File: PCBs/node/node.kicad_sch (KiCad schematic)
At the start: 13 parts, among them J1 Bat+, J2 GND, J3 5V, SW1 SW_Push, U1 ESP32-DEVKIT-V1, U2 BME280, U3 pm25sensor, U4 lidar

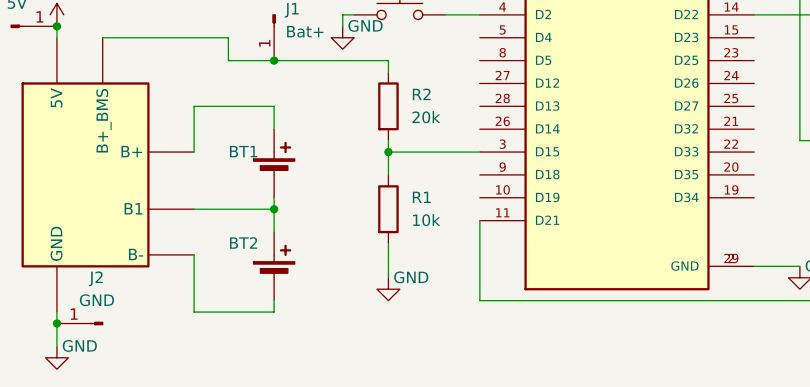
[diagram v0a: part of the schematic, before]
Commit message: changes
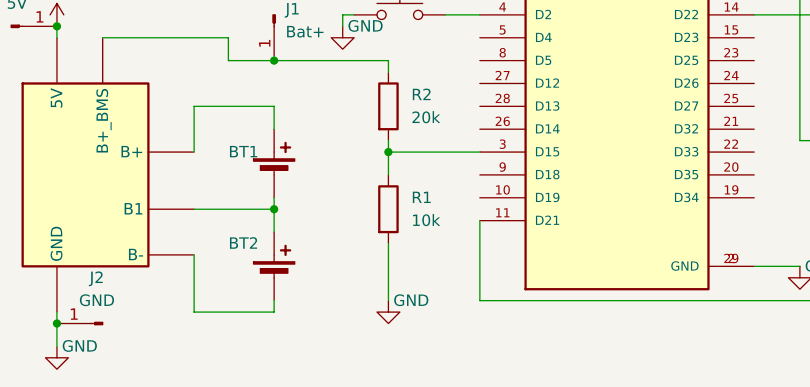
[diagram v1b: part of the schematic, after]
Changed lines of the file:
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@@
     (stroke (width 0) (type default))
   )
-  (wire (pts (xy 97.79 113.03) (xy 97.79 116.84))
+  (wire (pts (xy 97.79 113.03) (xy 97.79 119.38))
     (stroke (width 0) (type default))
   )
@@
     )
   )
-  (symbol (lib_id "power:GND") (at 97.79 116.84 0) (unit 1)
+  (symbol (lib_id "power:GND") (at 97.79 119.38 0) (unit 1)
     (in_bom yes) (on_board yes) (dnp no)
-    (property "Reference" "#PWR010" (at 97.79 123.19 0)
-      (effects (font (size 1.27 1.27)) hide)
-    )
-    (property "Value" "GND" (at 100.33 116.84 0)
-      (effects (font (size 1.27 1.27)))
-    )
-    (property "Footprint" "" (at 97.79 116.84 0)
-      (effects (font (size 1.27 1.27)) hide)
-    )
-    (property "Datasheet" "" (at 97.79 116.84 0)
-      (effects (font (size 1.27 1.27)) hide)
-    )
+    (property "Reference" "#PWR010" (at 97.79 125.73 0)
+      (effects (font (size 1.27 1.27)) hide)
+    )
+    (property "Value" "GND" (at 100.33 119.38 0)
+      (effects (font (size 1.27 1.27)))
+    )
+    (property "Footprint" "" (at 97.79 119.38 0)
+      (effects (font (size 1.27 1.27)) hide)
+    )
+    (property "Datasheet" "" (at 97.79 119.38 0)
+      (effects (font (size 1.27 1.27)) hide)
+    )

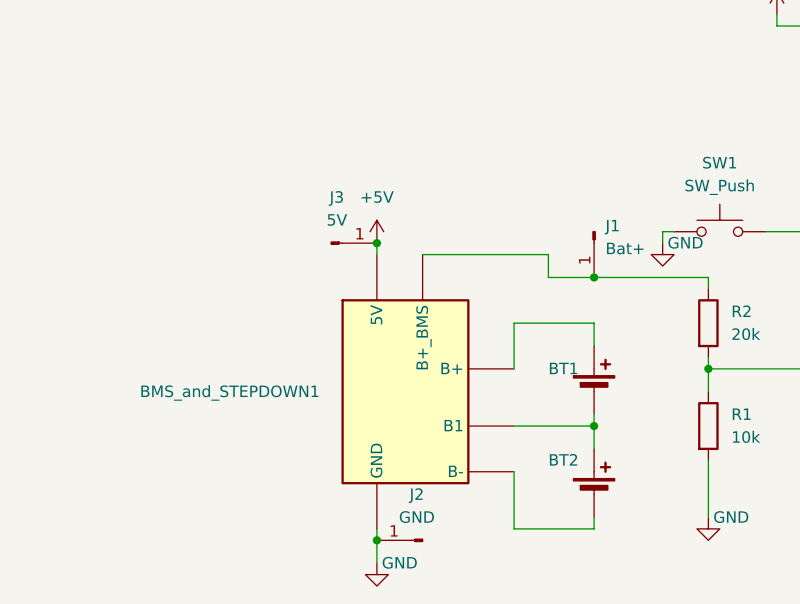
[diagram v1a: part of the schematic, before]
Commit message: changes
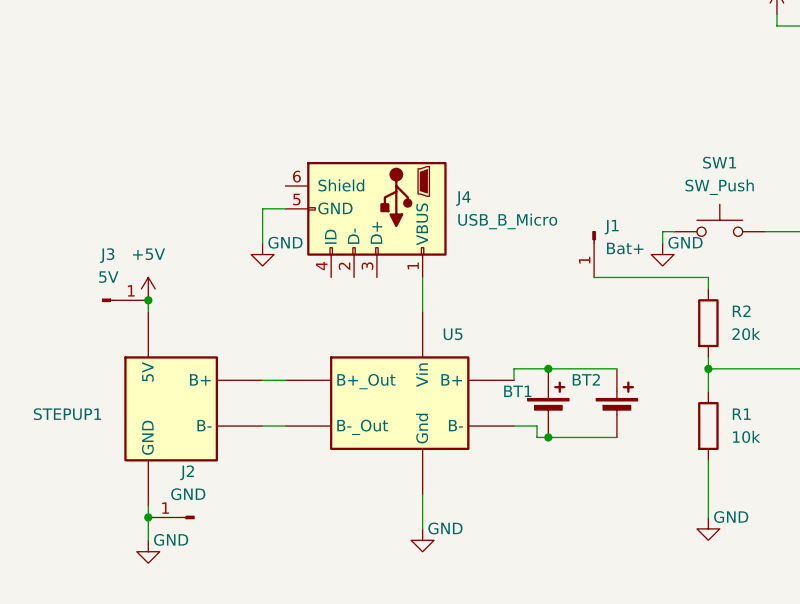
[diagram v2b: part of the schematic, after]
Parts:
- added J4: USB_B_Micro, symbol Connector:USB_B_Micro
- added U5: ~, symbol New_Library:BMS
- renumbered BMS_and_STEPDOWN1 to STEPUP1
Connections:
- net GND: now also J4.5 (GND), U5. (Vin)
- net at J1.1 (Pin_1), R2.1: no longer STEPUP1. (GND)
- net at BT1.1 (+): now also BT2.1 (+), U5. (Vin); no longer STEPUP1. (GND)
- net at BT2.2 (-): now also BT1.2 (-), U5. (Vin); no longer STEPUP1. (GND)
- new net: J4.1 (VBUS), U5. (Vin)
- new net: STEPUP1. (GND), U5. (Vin) (x2)
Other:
- moved on the sheet: BT1, BT2, J2, J3
